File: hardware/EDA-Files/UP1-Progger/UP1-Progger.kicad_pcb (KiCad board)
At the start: 2 copper layers, 29.2 x 35.2 mm, 16 parts, among them J1 UP1_Prog_Connector, J11 UP1_Prog_Connector, J2 USB_B_Micro, J3 Conn_01x03, J4 SWD_Interface, J5 ST Link V2 Clone, SW1 Reset, SW2 Bootsel, U1 LDO_3V3_SOT23-3

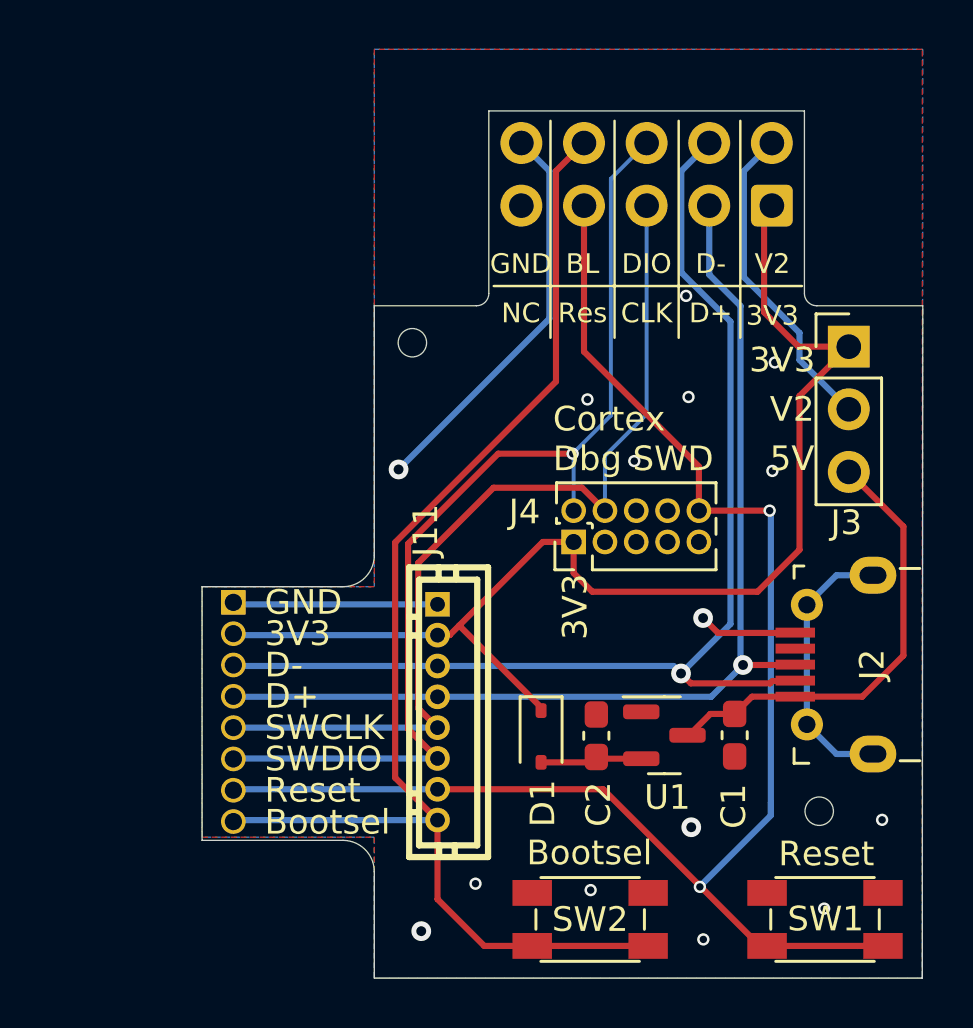
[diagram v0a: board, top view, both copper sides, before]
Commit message: UP1-Progger V02.00
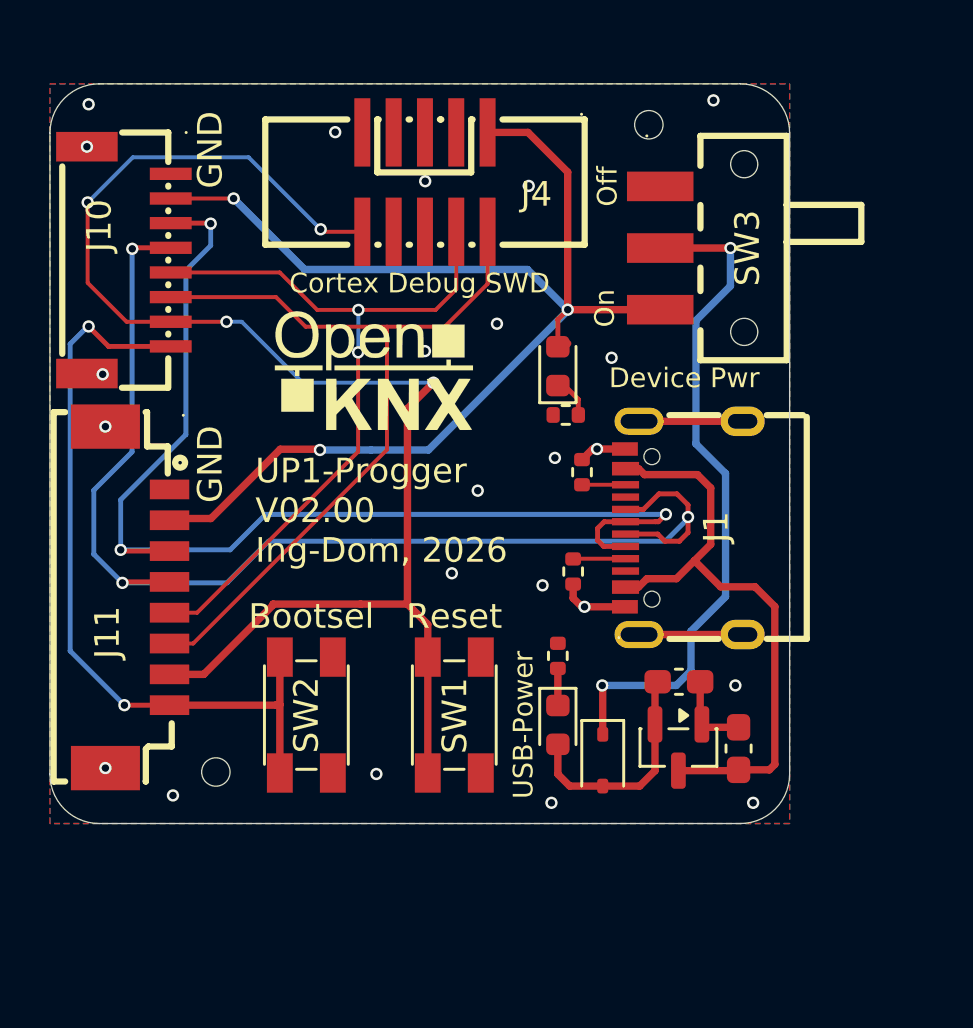
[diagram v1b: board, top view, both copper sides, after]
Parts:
- removed J2: USB_B_Micro, DomsKiCADLib:USB_Micro-B_JING_C10418
- removed J3: Conn_01x03, Connector_PinHeader_2.54mm:PinHeader_1x03_P2.54mm_Vertical
- removed J5: ST Link V2 Clone, Connector_IDC:IDC-Header_2x05_P2.54mm_Vertical
- removed the REF** at (115.2, 121.5)
- removed the REF** at (98.7, 102.5)
- added J10: UP1_Prog_125, EasyEDALib:CONN-SMD_8P-P1.00_MEGASTAR_ZX-SH1.0-8PWT, F.Cu at (87.2, 99.1)
- added LED1: USB-Power, Diode_SMD:D_0603_1608Metric, F.Cu at (104.6, 118.0)
- added LED2: Device_Pwr, Diode_SMD:D_0603_1608Metric, F.Cu at (104.6, 103.5)
- added R1: 2k, Resistor_SMD:R_0402_1005Metric, F.Cu at (104.6, 115.2)
- added R2: 2k, Resistor_SMD:R_0402_1005Metric, F.Cu at (104.9, 105.4)
- added R3: 5k1, Resistor_SMD:R_0402_1005Metric, F.Cu at (105.2, 111.8)
- added R4: 5k1, Resistor_SMD:R_0402_1005Metric, F.Cu at (105.6, 107.8)
- added REF**: JLCPCB_Tooling_hole, DomsKiCADLib:JLCPCB_Tooling_hole, F.Cu at (90.7, 119.9)
- added REF**: JLCPCB_Tooling_hole, DomsKiCADLib:JLCPCB_Tooling_hole, F.Cu at (108.3, 93.7)
- added SW3: SW_SPDT, EasyEDALib:SW-SMD_K3-1280S-K1, F.Cu at (112.2, 98.7)
- G***: moved to F.Cu
- J1: value UP1_Prog_Connector -> TYPE-C_16PIN_2MD(073); footprint Connector_PinSocket_1.27mm:PinSocket_1x08_P1.27mm_Vertical -> EasyEDALib:USB-C-SMD_TYPE-C-6PIN-2MD-073; moved to F.Cu
- J11: value UP1_Prog_Connector -> UP1_Prog_10; footprint EasyEDALib:CONN-TH_1.25-8A -> EasyEDALib:CONN-SMD_8P-P1.25-L4.4-W14.8
- J4: footprint Connector_PinHeader_1.27mm:PinHeader_2x05_P1.27mm_Vertical -> EasyEDALib:IDC-SMD_10P-P1.27-3220-10-0300-00
- moved J1 19.8 mm to (111.0, 110.0), turned to 90 degrees
- moved SW1 17.2 mm to (100.4, 117.6), turned to -90 degrees
- moved G*** 16.1 mm to (97.1, 103.6), turned to 0 degrees
- moved J4 15.8 mm to (99.2, 96.0), turned to 180 degrees
- moved SW2 14.2 mm to (94.4, 117.6), turned to -90 degrees
- moved G*** 14.0 mm to (98.0, 117.0)
- moved J11 13.0 mm to (87.5, 112.8)
- moved C2 4.00 mm to (109.5, 116.2), turned to 0 degrees
- moved D1 2.68 mm to (106.4, 119.4)
- moved U1 0.76 mm to (109.5, 118.9), turned to -90 degrees
- moved C1 0.57 mm to (111.9, 119.0), turned to 90 degrees
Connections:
- J1 pad 2: +3.3V -> +5V
- J1 pad 3: D- -> unconnected-(J1-SBU2-Pad3)
- J1 pad 4: D+ -> Net-(J1-CC1)
- J1 pad 5: SWCLK -> D-
- J1 pad 6: SWDIO -> D+
- J1 pad 7: Reset -> D-
- J1 pad 8: Bootsel -> D+
- J11 pad 2: +3.3V -> Net-(J10-3V3)
- J4 pad 1: +3.3V -> Net-(J10-3V3)
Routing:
- net Net-(J10-3V3): track 0.00 -> 52.8 mm, vias 0 -> 3
- net +3.3V: track 49.2 -> 27.5 mm, vias 0 -> 2
- net Bootsel: track 52.2 -> 31.3 mm, vias 0 -> 2
- net GND: track 28.5 -> 8.08 mm, vias 15 -> 23
- net Net-(J3-Pin_2): track 13.0 -> 0.00 mm
- net unconnected-(J2-Shield-Pad6): track 11.2 -> 0.00 mm
- net SWDIO: track 41.8 -> 33.2 mm, vias 1 -> 0
- net D+: track 42.5 -> 49.2 mm, vias 1 -> 3
- net SWCLK: track 37.6 -> 31.0 mm, vias 0 -> 2
- net +5V: track 18.4 -> 24.7 mm
- net Net-(D1-A): track 4.12 -> 9.26 mm
- net unconnected-(J1-SHELL-Pad14): track 0.00 -> 4.20 mm
- net unconnected-(J1-SHELL-Pad13): track 0.00 -> 4.20 mm
- net Reset: track 63.1 -> 59.6 mm, vias 2 -> 4
- net Net-(J1-CC1): track 0.00 -> 2.13 mm
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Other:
- board size 29.2 x 35.2 mm -> 30 x 30 mm
- board text added: "Cortex Debug SWD"
- board text added: "Device Pwr"
- board text added: "Off"
- board text added: "On"
- board text added: "UP1-Progger V02.00 Ing-Dom, 2026"
- board text removed: "3V3"
- board text removed: "5V"
- board text removed: "BL"
- board text removed: "Bootsel"
- board text removed: "CLK"
- board text removed: "Cortex Dbg SWD"
- board text removed: "D+"
- board text removed: "D-"
- board text removed: "DIO"
- board text removed: "NC"
- board text removed: "Res"
- board text removed: "Reset"
- board text removed: "SWCLK"
- board text removed: "SWDIO"
- board text removed: "UP1-Progger V01.10 by Ing-Dom, 2024"
- board text removed: "V2"
